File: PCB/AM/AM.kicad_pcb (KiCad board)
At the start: 2 copper layers, 30.5 x 30.5 mm, 10 parts, among them J4 Conn_01x05

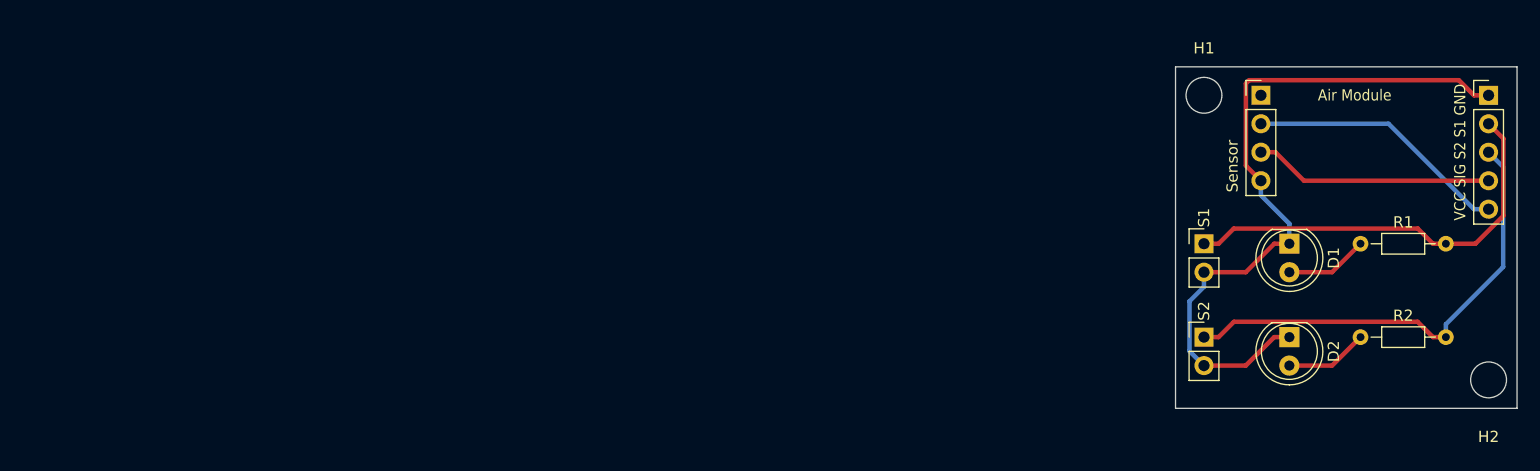
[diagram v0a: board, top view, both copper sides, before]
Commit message: Flere billedere
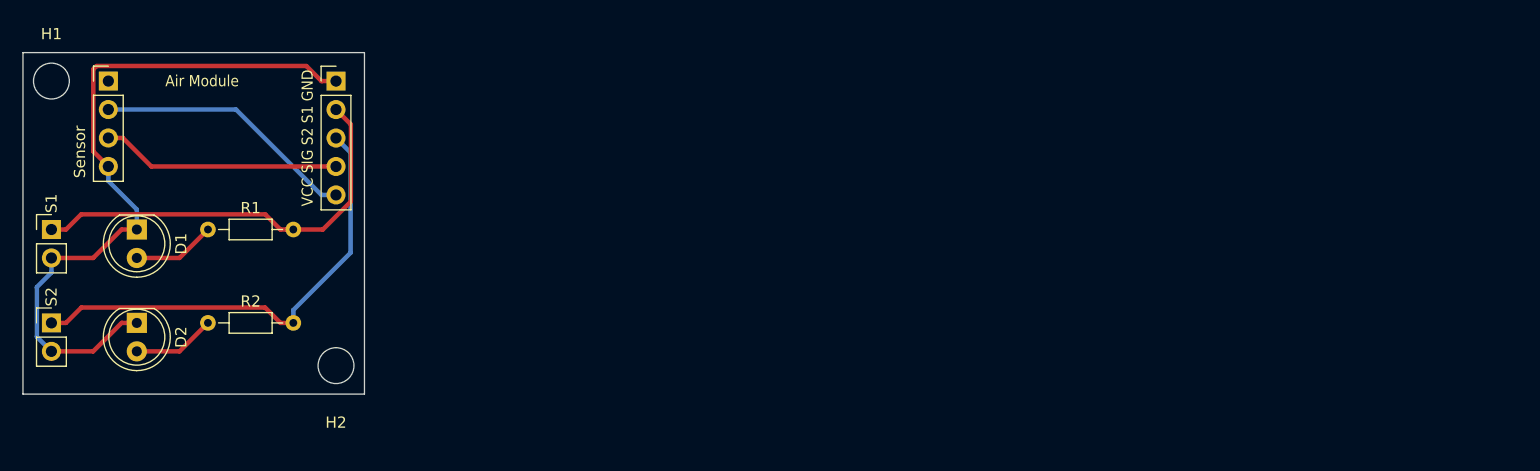
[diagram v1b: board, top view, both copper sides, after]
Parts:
- moved D1 102.9 mm to (69.8, 93.3)
- moved D2 102.9 mm to (69.8, 101.6)
- moved H1 102.9 mm to (62.2, 80.0)
- moved H2 102.9 mm to (87.6, 105.4)
- moved J4 102.9 mm to (87.6, 80.0)
- moved S1 102.9 mm to (62.2, 93.3)
- moved S2 102.9 mm to (62.2, 101.6)
- moved Sensor 102.9 mm to (67.3, 80.0)
- moved R1 102.9 mm to (76.2, 93.3)
- moved R2 102.9 mm to (76.2, 101.6)
